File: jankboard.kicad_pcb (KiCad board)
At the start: 2 copper layers, 152.4 x 85.7 mm, 157 parts, among them J1 F31L-1A7H1-11030, J2 F31L-1A7H1-11030, J3 Conn_01x02, J4 Conn_01x02, J5 Conn_01x04_Pin, SW1 SW_Push_45deg, SW10 SW_Push_45deg, SW11 SW_Push_45deg, SW12 SW_Push_45deg, SW13 SW_Push_45deg, SW14 SW_Push_45deg, SW15 SW_Push_45deg, SW16 SW_Push_45deg, SW17 SW_Push_45deg, SW18 SW_Push_45deg, SW19 SW_Push_45deg, SW2 SW_Push_45deg, SW20 SW_Push_45deg, SW21 SW_Push_45deg, SW3 SW_Push_45deg, SW4 SW_Push_45deg, SW5 SW_Push_45deg, SW6 SW_Push_45deg, SW7 SW_Push_45deg, SW8 SW_Push_45deg, SW9 SW_Push_45deg, U1 nice_nano

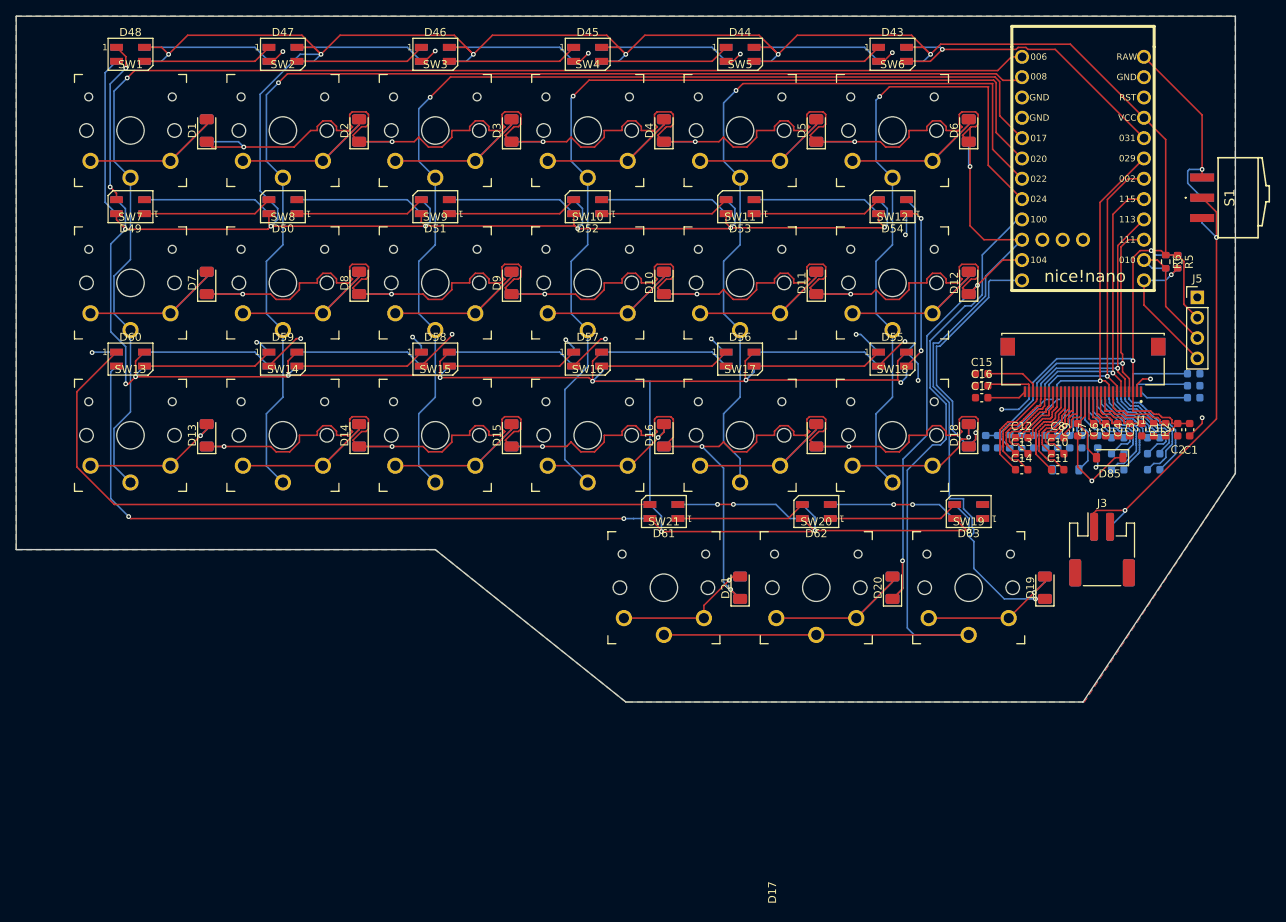
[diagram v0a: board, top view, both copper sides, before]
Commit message: add led switch
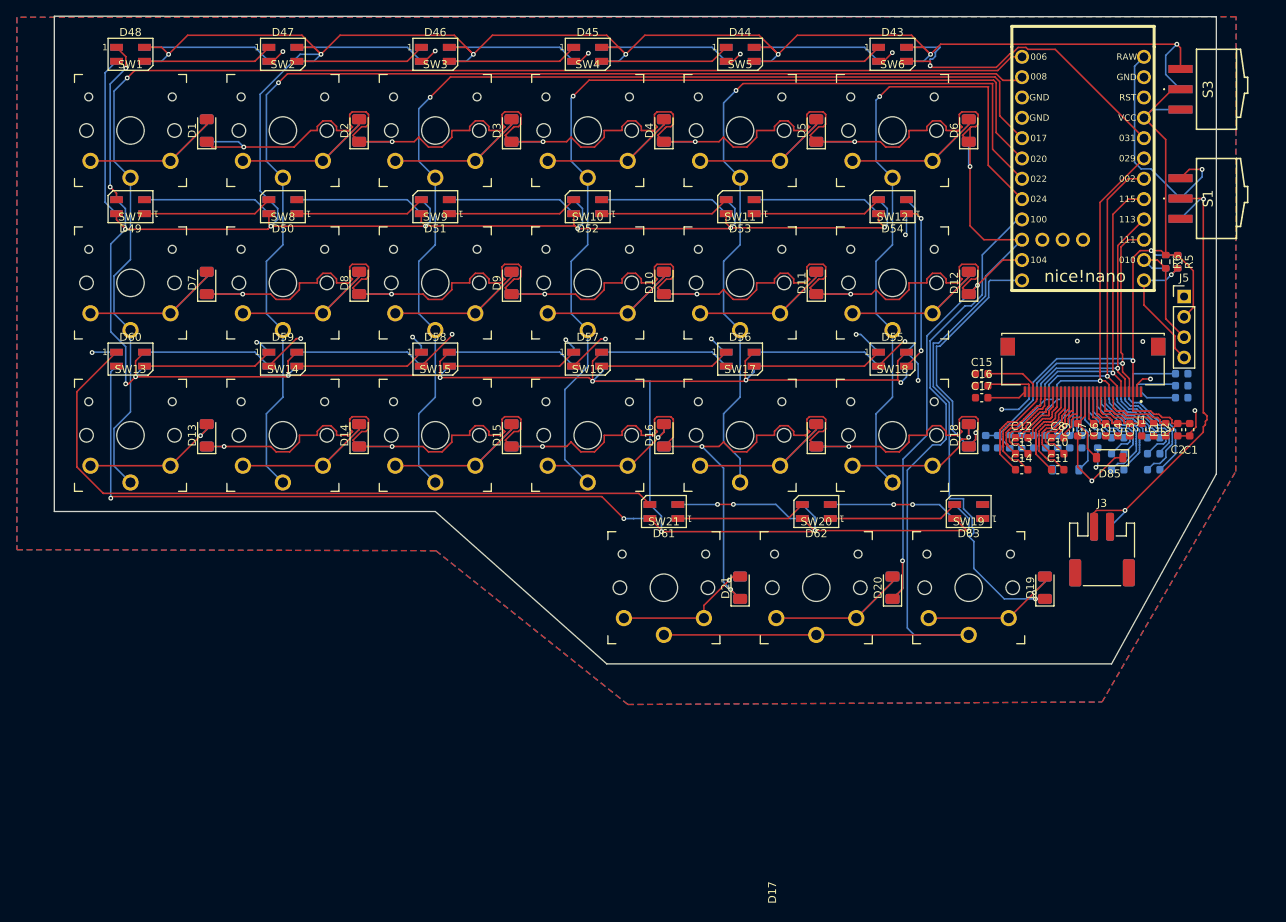
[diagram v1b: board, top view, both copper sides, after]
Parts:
- added S3: EGJ1210AAG2R, KiCad:EGJ1210AAG2R, F.Cu at (173.6, 33.0)
- added S4: EGJ1210AAG2R, KiCad:EGJ1210AAG2R, B.Cu at (173.6, 33.0)
- moved S1 2.70 mm to (173.6, 46.6)
- moved S2 2.70 mm to (173.6, 46.6)
- moved J5 1.65 mm to (169.8, 58.9)
- moved C32 1.50 mm to (169.5, 68.5)
- moved C33 1.50 mm to (169.5, 70.0)
- moved C34 1.50 mm to (169.5, 71.5)
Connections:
- D43 pad 4: +3.3V -> NP
- D44 pad 4: +3.3V -> NP
- D45 pad 4: +3.3V -> NP
- D46 pad 4: +3.3V -> NP
- D47 pad 4: +3.3V -> NP
- D48 pad 4: +3.3V -> NP
- D49 pad 4: +3.3V -> NP
- D50 pad 4: +3.3V -> NP
- D51 pad 4: +3.3V -> NP
- D52 pad 4: +3.3V -> NP
- D53 pad 4: +3.3V -> NP
- D54 pad 4: +3.3V -> NP
- D55 pad 4: +3.3V -> NP
- D56 pad 4: +3.3V -> NP
- D57 pad 4: +3.3V -> NP
- D58 pad 4: +3.3V -> NP
- D59 pad 4: +3.3V -> NP
- D60 pad 4: +3.3V -> NP
- D61 pad 4: +3.3V -> NP
- D62 pad 4: +3.3V -> NP
- D63 pad 4: +3.3V -> NP
- D64 pad 4: +3.3V -> NP
- D65 pad 4: +3.3V -> NP
- D66 pad 4: +3.3V -> NP
- D67 pad 4: +3.3V -> NP
- D68 pad 4: +3.3V -> NP
- D69 pad 4: +3.3V -> NP
- D70 pad 4: +3.3V -> NP
- D71 pad 4: +3.3V -> NP
- D72 pad 4: +3.3V -> NP
- D73 pad 4: +3.3V -> NP
- D74 pad 4: +3.3V -> NP
- D75 pad 4: +3.3V -> NP
- D76 pad 4: +3.3V -> NP
- D77 pad 4: +3.3V -> NP
- D78 pad 4: +3.3V -> NP
- D79 pad 4: +3.3V -> NP
- D80 pad 4: +3.3V -> NP
- D81 pad 4: +3.3V -> NP
- D82 pad 4: +3.3V -> NP
- D83 pad 4: +3.3V -> NP
- D84 pad 4: +3.3V -> NP
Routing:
- net NP: track 0.00 -> 577.8 mm, vias 0 -> 23
- net +3.3V: track 659.5 -> 103.6 mm, vias 24 -> 2
- net Net-(S1-NO): track 24.0 -> 29.2 mm
- net NEO: track 39.7 -> 43.3 mm
- net Net-(J3-Pin_1): track 56.3 -> 58.8 mm
- net GND: track 75.0 -> 76.9 mm, vias 21 -> 23
- net Net-(C34-Pad2): track 6.12 -> 4.62 mm
- net Net-(C33-Pad2): track 7.26 -> 5.76 mm
- net Net-(C32-Pad2): track 9.08 -> 7.58 mm
- net SCL: track 16.6 -> 15.8 mm
- net SDA: track 18.5 -> 17.7 mm
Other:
- board size 152.4 x 85.7 mm -> 145.3 x 81 mm
